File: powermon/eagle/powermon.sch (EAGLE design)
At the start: 25 parts, among them J1 USBSMD, J3 USBSMD, U1 LTC2290, U2 FT232RL, U3 ATMEGA328, X1 16MHz

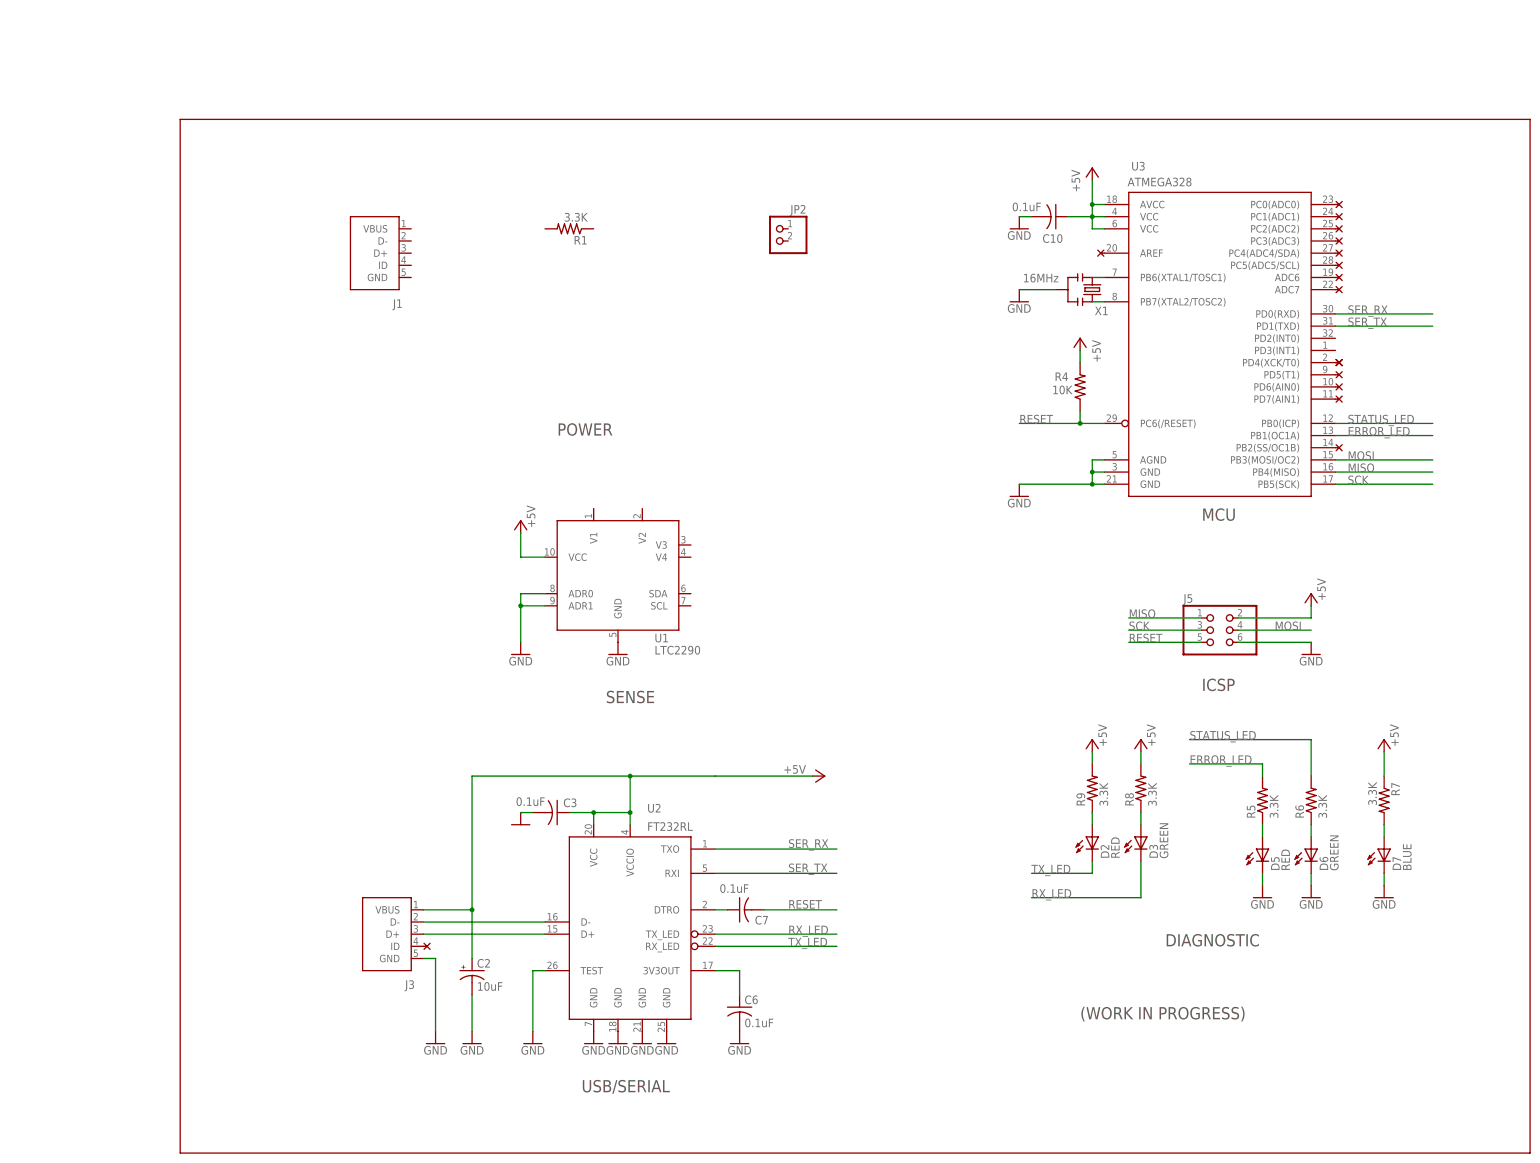
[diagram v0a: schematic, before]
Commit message: Updated schematic.
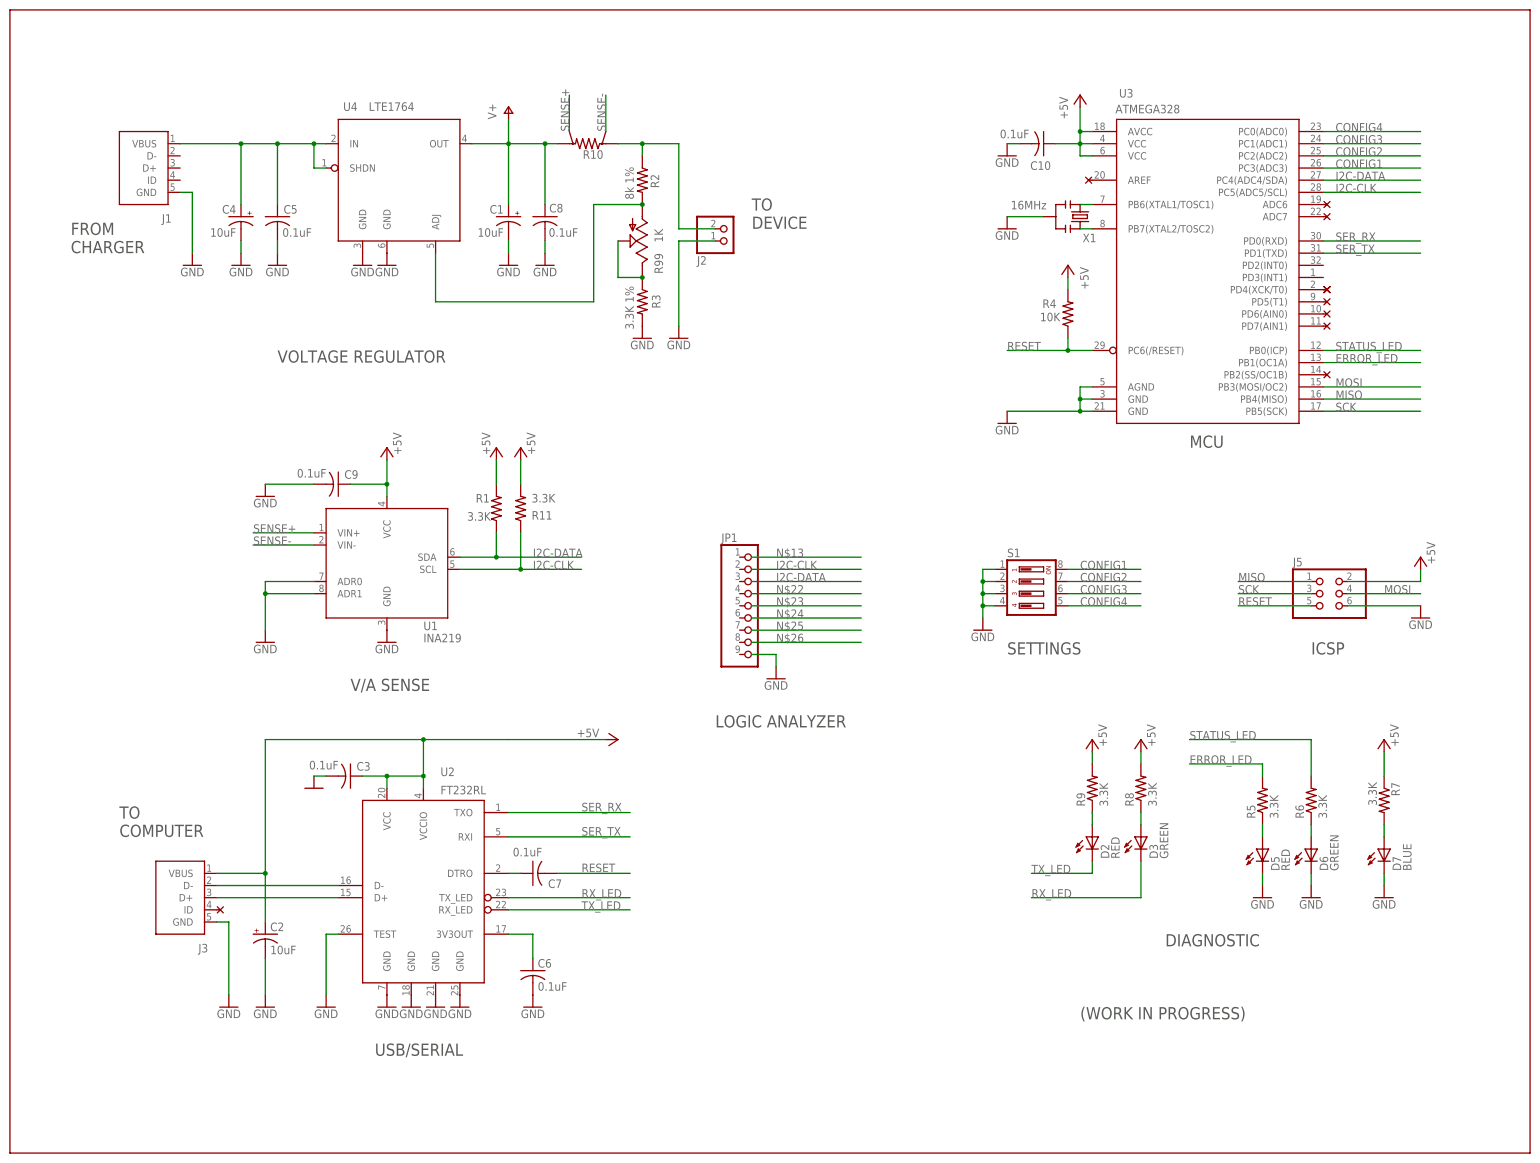
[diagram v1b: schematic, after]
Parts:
- removed JP2: (no value), powermon:PINHD-1X2
- added C1, C4: 10uF, powermon:CPOL-USA/3216-18R
- added C5, C8, C9: 0.1uF, powermon:C-USC0805
- added J2: TERMINAL-2, powermon:TERMINAL-2
- added JP1: (no value), powermon:PINHD-1X9
- added R10: (no value), powermon:SHUNT
- added R11: 3.3K, powermon:R-US_R0805
- added R2: 8k 1%, powermon:R-US_R0805
- added R3: 3.3K 1%, powermon:R-US_R0805
- added R99: 1K, powermon:TRIM_US-SM-42/43A
- added S1: 219-04, powermon:219-04
- added U4: LTE1764, powermon:LTE1764
- U1: value LTC2290 -> INA219; device powermon:LTC2290 -> powermon:INA219
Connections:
- new net CONFIG1: S1.8, U3.PC3(ADC3)
- new net CONFIG2: S1.7, U3.PC2(ADC2)
- new net CONFIG3: S1.6, U3.PC1(ADC1)
- new net CONFIG4: S1.5, U3.PC0(ADC0)
- new net I2C-CLK: R11.1, U1.SCL, U3.PC5(ADC5/SCL)
- new net I2C-DATA: R1.1, U1.SDA, U3.PC4(ADC4/SDA)
- new net N$18: R3.1, R99.E, R99.S
- new net N$19: R2.2, R99.A, U4.ADJ
- new net N$5: J2.2, R10.I1, R2.1
- new net N$9: C4.+, C5.1, J1.VBUS, U4.IN, U4.SHDN
- new net SENSE+: R10.V2, U1.VIN+
- new net SENSE-: R10.V1, U1.VIN-
- new net V+: C1.+, C8.1, R10.I2, U4.OUT
- net +5V: now also C9.1, R1.2, R11.2
- net GND: now also C1.-, C4.-, C5.2, C8.2, C9.2, J1.GND, J2.1, R3.2, S1.1, S1.2, S1.3, S1.4, U4.GND@1, U4.GND@2
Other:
- note added: "FROM CHARGER"
- note added: "LOGIC ANALYZER"
- note added: "SETTINGS"
- note added: "TO COMPUTER"
- note added: "TO DEVICE"
- note added: "V/A SENSE"
- note added: "VOLTAGE REGULATOR"
- note removed: "POWER"
- note removed: "SENSE"
- moved on the sheet: C10, C2, C3, C6, C7, J1, J3, J5, R1, R4, U2, U3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
